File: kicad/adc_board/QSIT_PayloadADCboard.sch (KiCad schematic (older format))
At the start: 61 parts, among them J1 Conn_01x09, J2 Power_Conn, J4 Conn_ARM_JTAG_SWD_10, J5 Conn_01x03, J6 Conn_02x05_Odd_Even, SW1 SW_Push, U1 MCP3564, U2 MAX6070, U3 STM32F373CCT6, U4 TC1108-3.3VDBTR, U5 MPE1205S-1W, X1 ECS-2520MVLC-049-BN, Y1 Crystal_GND24

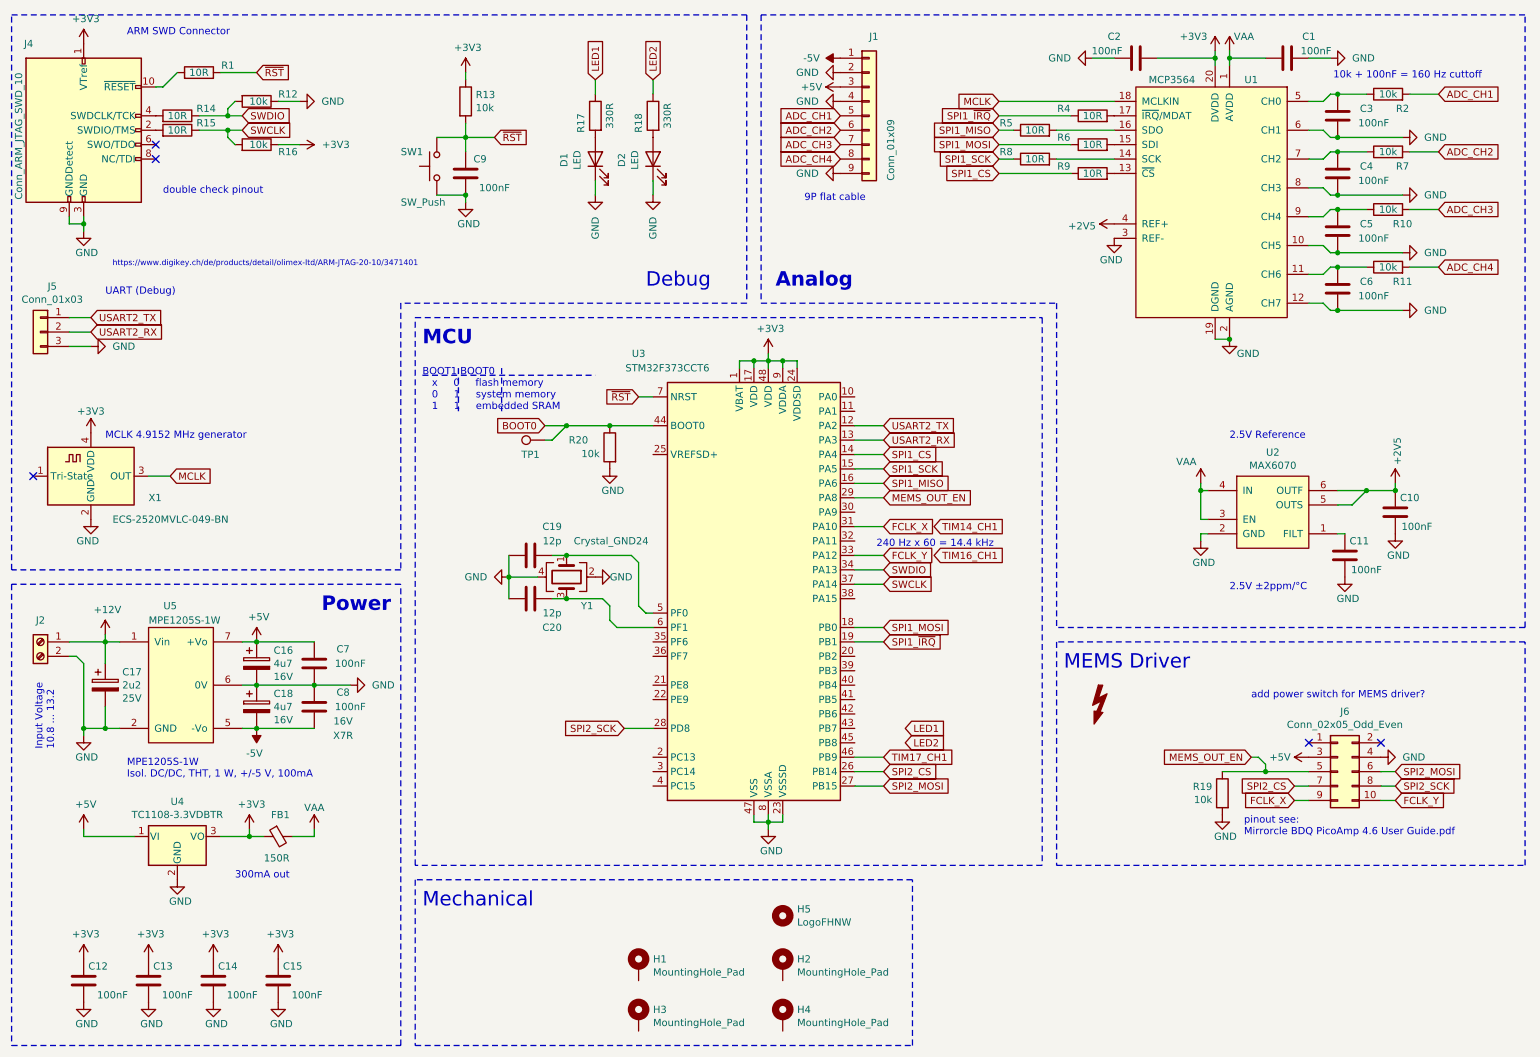
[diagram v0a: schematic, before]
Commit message: further pcb improvements
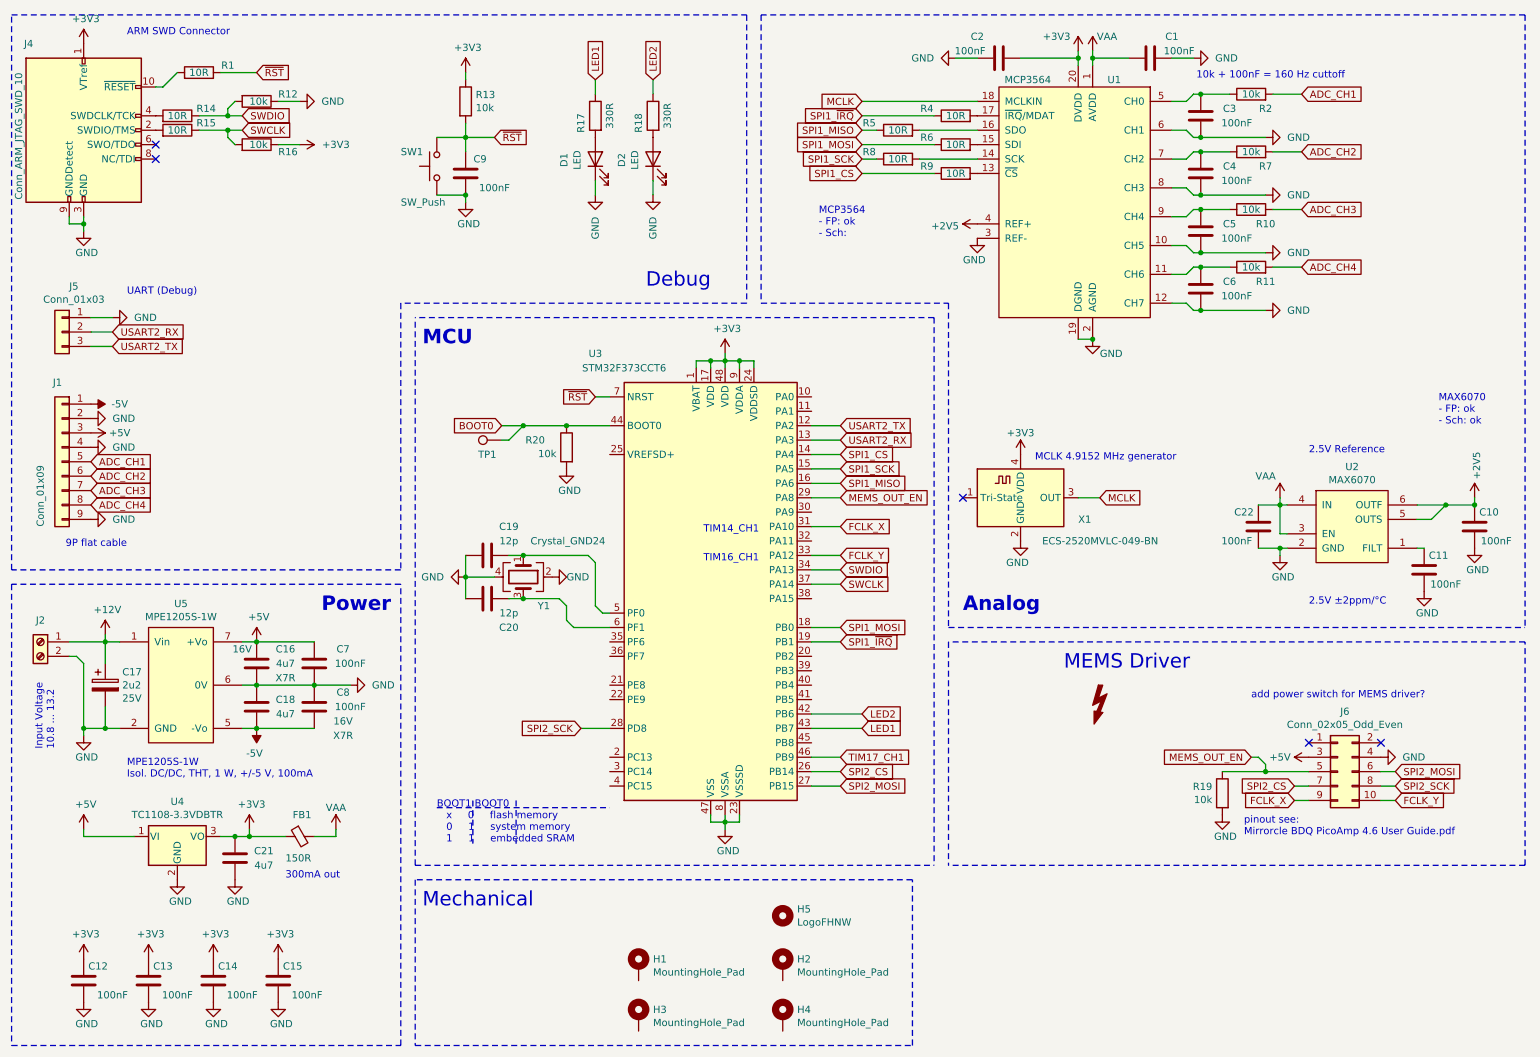
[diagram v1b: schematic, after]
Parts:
- removed C16, C18: 4u7, Capacitor_THT:CP_Radial_D4.0mm_P2.00mm, symbol Device:CP
- removed U1: MCP3564, Package_SO:TSSOP-20_4.4x6.5mm_P0.65mm, symbol A_Tale_Of_A_Library:MCP3564
- removed U2: MAX6070, Package_TO_SOT_SMD:SOT-23-6_Handsoldering, symbol A_Tale_Of_A_Library:MAX6070
- removed U5: MPE1205S-1W, A_Tale_Of_A_Library:Converter_DCDC_multicorp_THT, symbol A_Tale_Of_A_Library:MPE1205S-1W
- added C16, C18, C21: 4u7, Capacitor_SMD:C_1206_3216Metric, symbol Device:C
- added C22: 100nF, Capacitor_SMD:C_0603_1608Metric, symbol Device:C
- added U1: MCP3564, Package_SO:TSSOP-20_4.4x6.5mm_P0.65mm, symbol simonmartin_kicad_lib:MCP3564
- added U2: MAX6070, Package_TO_SOT_SMD:SOT-23-6_Handsoldering, symbol simonmartin_kicad_lib:MAX6070
- added U5: MPE1205S-1W, simonmartin_kicad_lib:Converter_DCDC_multicorp_THT, symbol simonmartin_kicad_lib:MPE1205S-1W
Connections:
- net +12V: now also U5.1 (Vin)
- net +2V5: now also U1.4 (REF+), U2.5 (OUTS), U2.6 (OUTF)
- net +3V3: now also C21.2, U1.20 (DVDD)
- net +5V: now also C16.2, U5.7 (+Vo)
- net -5V: now also C18.1, U5.5 (-Vo)
- net GND: now also J5.1 (Pin_1), C16.1, C18.2, C21.1, C22.1, U1.10 (CH5), U1.12 (CH7), U1.19 (DGND), U1.2 (AGND), U1.3 (REF-), U1.6 (CH1), U1.8 (CH3), U2.2 (GND), U5.2 (GND), U5.6 (0V); no longer J5.3 (Pin_3)
- net LED1: now also U3.43 (PB7)
- net LED2: now also U3.42 (PB6)
- net MCLK: now also U1.18 (MCLKIN)
- net USART2_TX: now also J5.3 (Pin_3); no longer J5.1 (Pin_1)
- net VAA: now also C22.2, U1.1 (AVDD), U2.3 (EN), U2.4 (IN)
- net at C3.2, R2.1: now also U1.5 (CH0)
- net at C4.2, R7.1: now also U1.7 (CH2)
- net at C5.2, R10.1: now also U1.9 (CH4)
- net at C6.2, R11.1: now also U1.11 (CH6)
- net at R9.2: now also U1.13 (~CS~)
- net at R8.2: now also U1.14 (SCK)
- net at R6.2: now also U1.15 (SDI)
- net at R5.2: now also U1.16 (SDO)
- net at R4.2: now also U1.17 (~IRQ~/MDAT)
- net at C11.2: now also U2.1 (FILT)
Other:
- note added: "MAX6070\n- FP: ok\n- Sch: ok"
- note added: "MCP3564\n- FP: ok\n- Sch:"
- note added: "TIM14_CH1"
- note added: "TIM16_CH1"
- note removed: "240 Hz x 60 = 14.4 kHz"
- note removed: "double check pinout"
- note removed: "https://www.digikey.ch/de/products/detail/olimex-ltd/ARM-JTAG-20-10/3471401"
- moved on the sheet: C1, C10, C11, C19, C2, C20, C3, C4, C5, C6, FB1, J1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

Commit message: rev.1 of ADC board
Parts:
- J6: footprint Connector_PinSocket_1.27mm:PinSocket_2x05_P1.27mm_Vertical_SMD -> Connector_PinHeader_1.27mm:PinHeader_2x05_P1.27mm_Vertical_SMD
